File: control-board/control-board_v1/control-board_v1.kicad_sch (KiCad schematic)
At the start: 57 parts, among them J1 Barrel_Jack, J2 Header-M_2x6, J3 Header-M_2x6, J4 Header-M_2x6, J5 Header-M_2x6, J6 Header_1x8, J7 Header_1x8, J8 Header_1x10, J9 Header_1x8, Q1 PMOS, Q2 PMOS, Q3 PMOS, Q4 PMOS, Q5 PMOS, Q6 PMOS, Q7 PMOS, Q8 PMOS, U1 CD74HCT154M

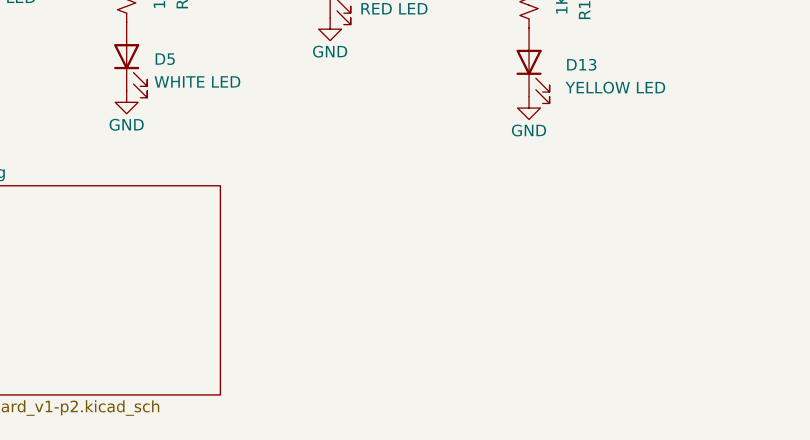
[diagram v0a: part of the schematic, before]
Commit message: additional notes
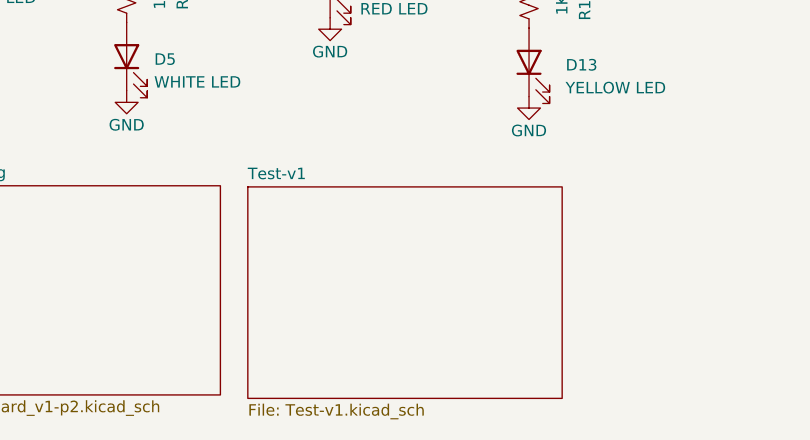
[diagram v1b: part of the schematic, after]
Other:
- added sheet Test-v1 (Test-v1.kicad_sch)
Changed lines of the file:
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@@
+    )
+  )
+  (sheet (at 56.134 169.037) (size 34.925 23.495) (fields_autoplaced)
+    (stroke (width 0.1524) (type solid))
+    (fill (color 0 0 0 0.0000))
+    (property "Sheetname" "Test-v1" (at 56.134 168.3254 0)
+      (effects (font (size 1.27 1.27)) (justify left bottom))
+    )
+    (property "Sheetfile" "Test-v1.kicad_sch" (at 56.134 193.1166 0)
+      (effects (font (size 1.27 1.27)) (justify left top))
+    )
+    (instances
+      (project "control-board_v1"
+        (path "/5ea0e920-d127-456d-9ad4-df9bbc649b9b" (page "3"))
+      )
     )
   )
